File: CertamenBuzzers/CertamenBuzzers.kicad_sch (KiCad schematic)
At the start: 65 parts, among them J1 USB_C_Receptacle_USB2.0_14P, J10 C4, J11 B4, J12 A4, J14 C1, J2 B1, J3 A1, J4 C2, J5 B2, J6 A2, J7 A3, J8 B3, J9 C3, SW1 BOOT, SW2 RST, SW3 SW_Push, SW4 Score_{A}, SW5 Score_{A}, SW6 Score_{A}, U1 RP2040, U2 NCP1117-3.3_SOT223, U3 TVS1400DRV, U4 W25Q32JVZP, Y1 12MHz

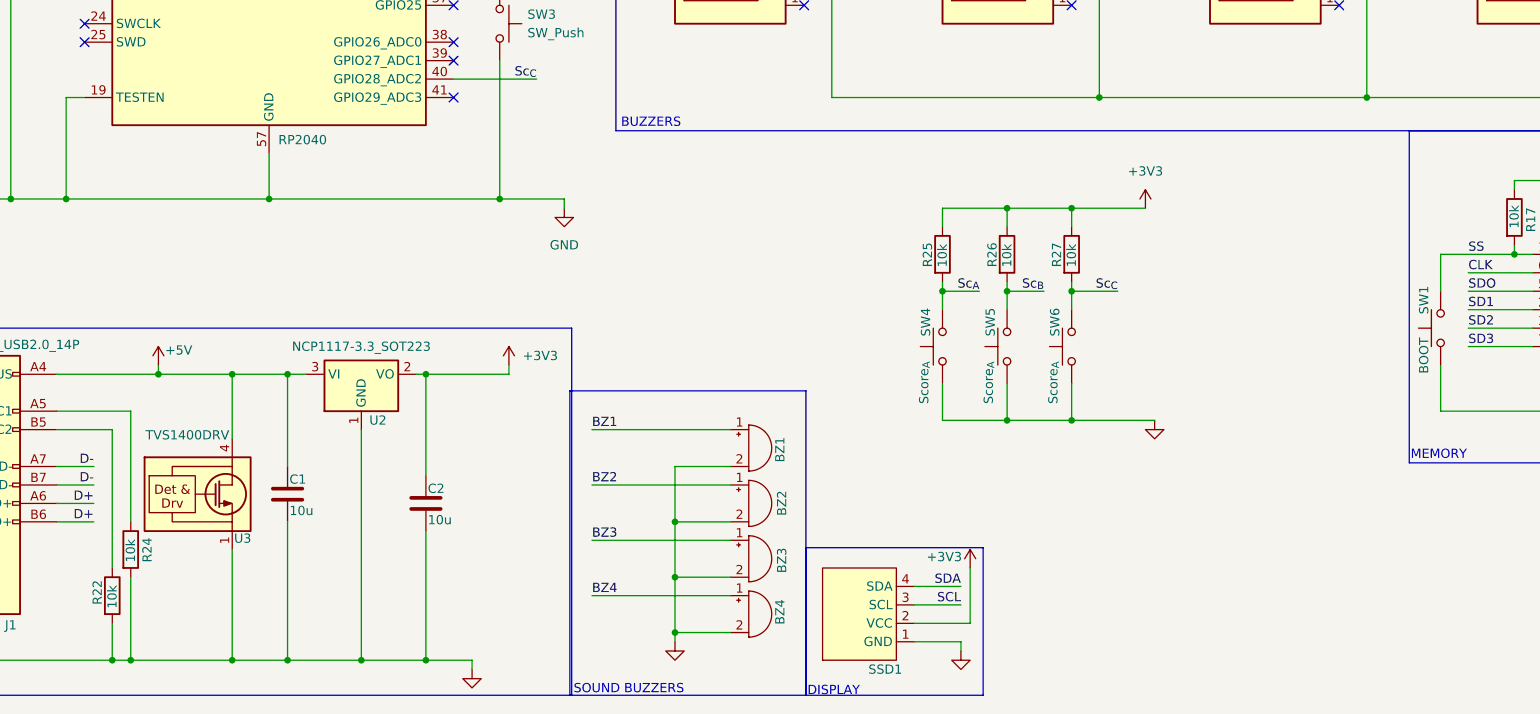
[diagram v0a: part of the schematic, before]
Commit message: code button stuff
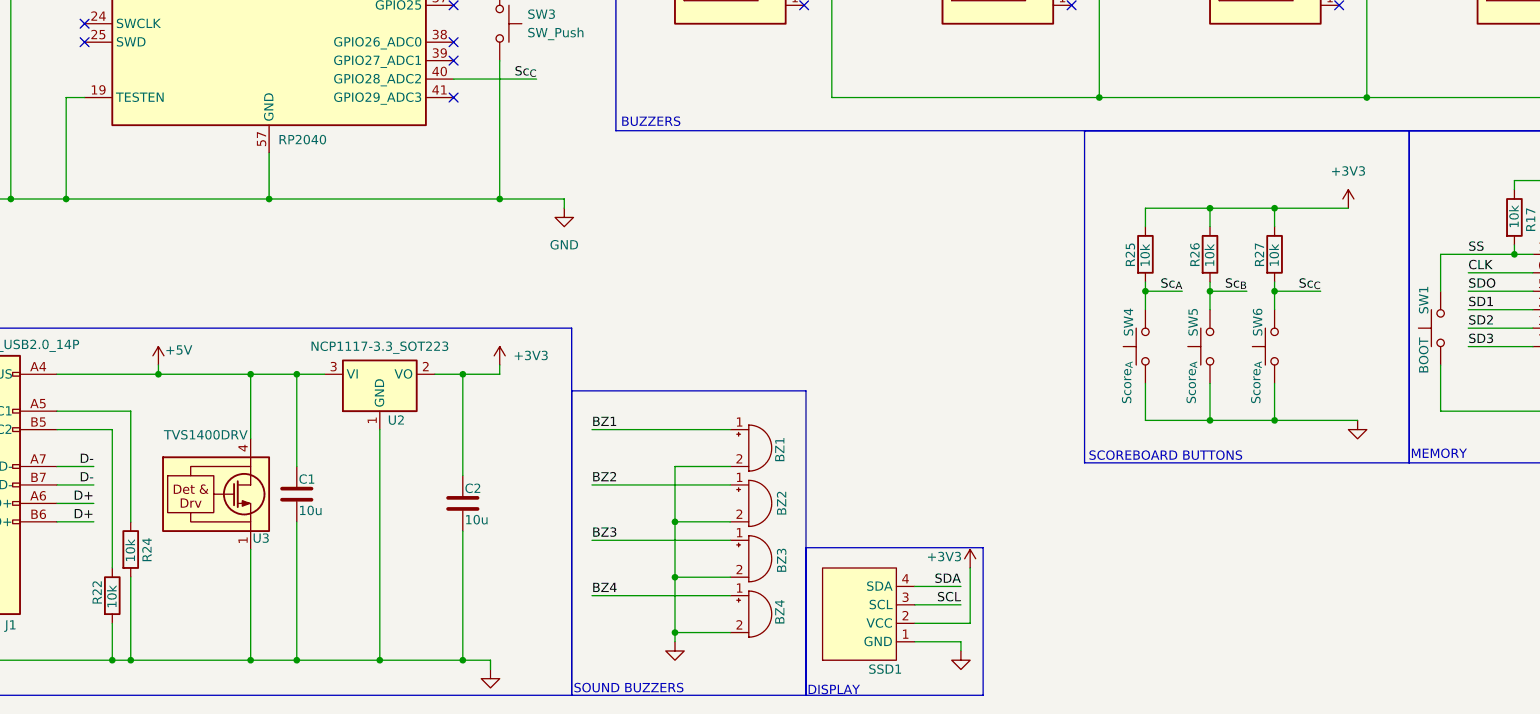
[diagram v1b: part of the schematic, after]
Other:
- note added: "SCOREBOARD BUTTONS"
- moved on the sheet: C1, C2, R25, R26, R27, SW4, SW5, SW6, U2, U3
